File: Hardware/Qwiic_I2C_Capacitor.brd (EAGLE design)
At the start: 25.4 x 25.4 mm, 38 parts, among them J2 QWIIC_RIGHT_ANGLE, J3 PTH, J4 QWIIC_RIGHT_ANGLE, U1 NCD2400MDFN

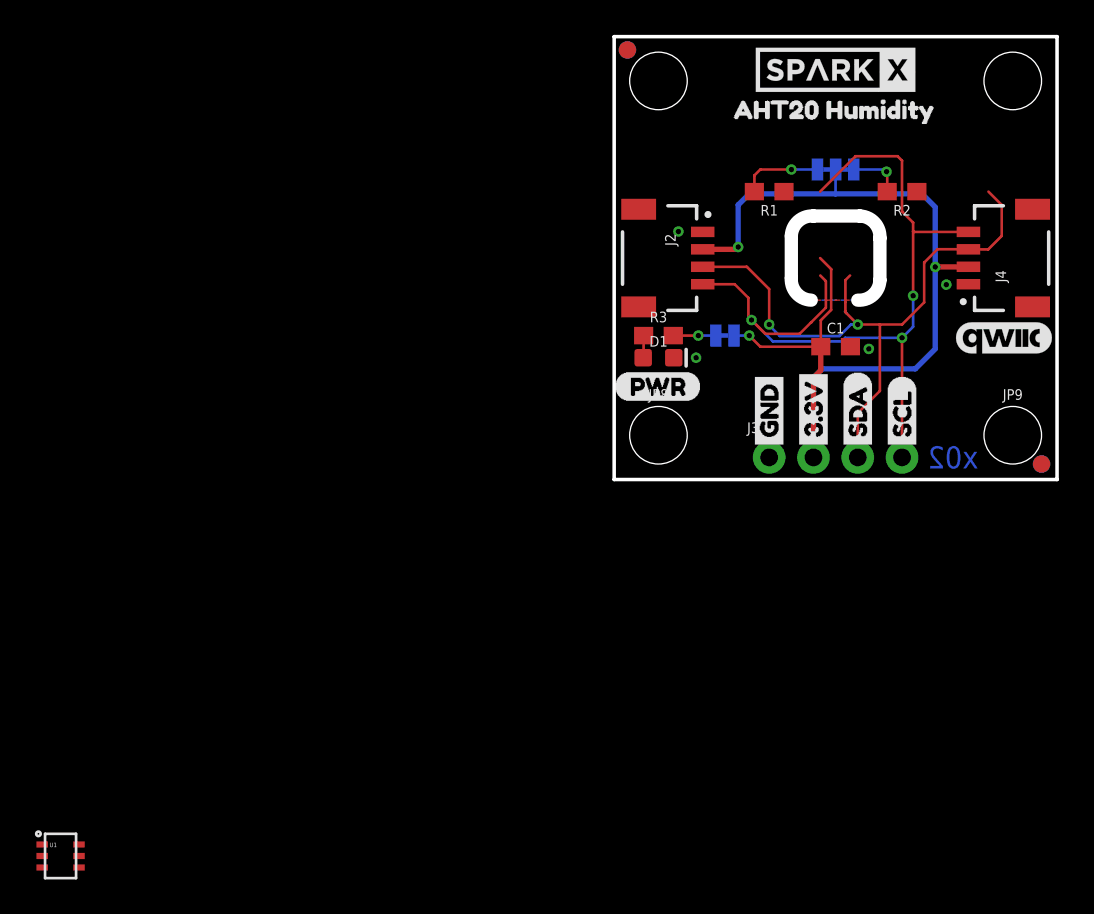
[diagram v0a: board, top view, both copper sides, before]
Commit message: Initial layout
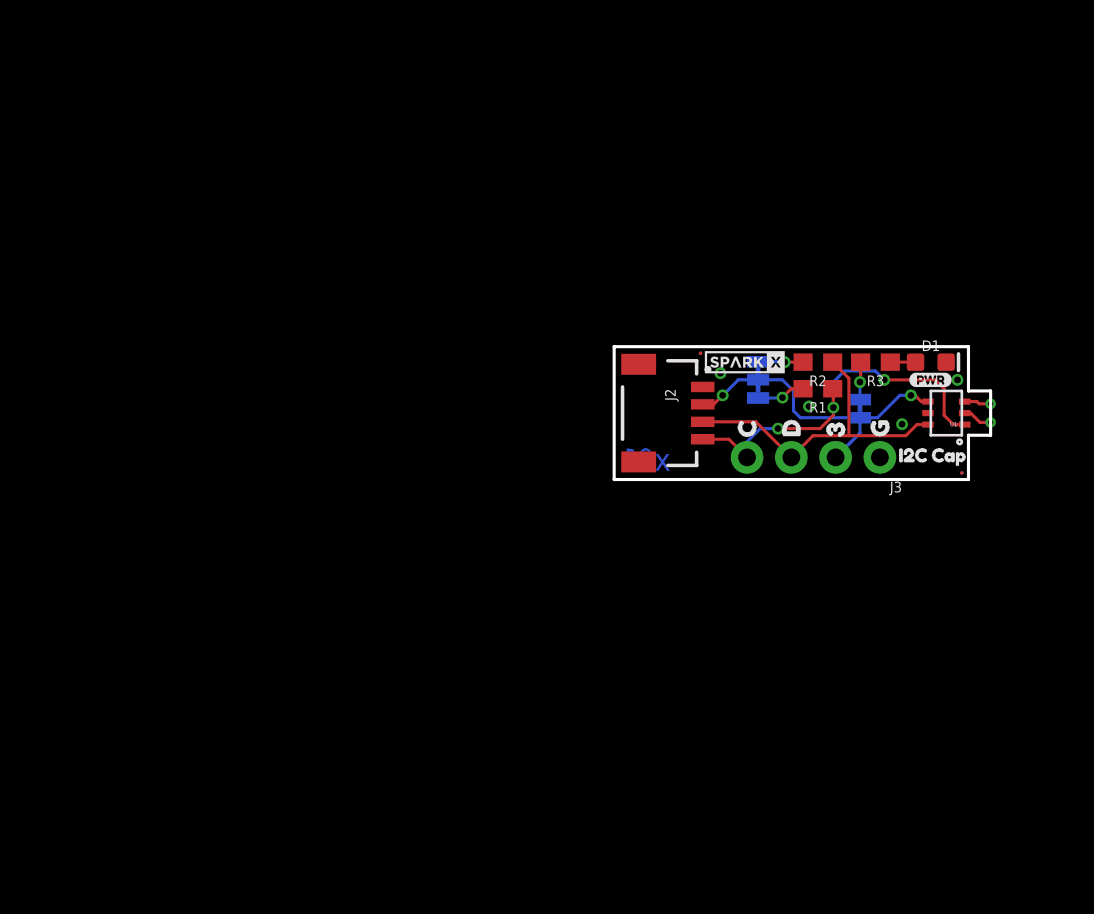
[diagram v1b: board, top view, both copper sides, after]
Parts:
- removed C1: 0.1uF, SparkFun-Capacitors:0603
- removed J4: QWIIC_RIGHT_ANGLE, SparkFun-Connectors:JST04_1MM_RA
- removed JP3, JP4, JP8, JP9: STAND-OFF, SparkFun-Hardware:STAND-OFF
- removed U$11: (no value), SparkFun-Aesthetics:QWIIC_5.5MM
- removed U$22: (no value), Labels-0_04:GND1
- removed U$26: (no value), Labels-0_04:SCL9
- removed U$27: (no value), Labels-0_04:SDA8
- added J1: CONN_02_0603, Qwiic_Capacitor:0603_CASTELLATED
- added U$13: (no value), buzzard_labels (81):D1
- added U$15: (no value), buzzard_labels (83):LED0
- added U$16: (no value), SparkX:SPARKX-TINY
- added U$17: (no value), buzzard_labels (86):CAP1
- added U$19: (no value), buzzard_labels (86):I2C0
- added U$20: (no value), Labels:QWIIC_COPYRIGHT_SMALL
- added U$7: (no value), buzzard_labels (81):32
- JP1, JP2, JP5, JP6: value FIDUCIAL1X2 -> FIDUCIAL0.2MM; device SparkFun-Aesthetics:FIDUCIAL-1X2 -> SparkFun-Aesthetics:FIDUCIAL-0.2MM
- U$1: value SPARKX-LOGO4 -> (none); device SparkX:SPARKX-MEDIUM -> buzzard_labels (86):I2C0
- U$10: device Labels-0_04:(PWR) -> buzzard_labels (85):PWR0
- U$12: device SparkFun-Buzzard:LED_32 -> SparkX:SPARKX-TINY
- U$14: device buzzard_labels (17):AHT20_HUMIDITY2 -> buzzard_labels (81):G3
- U$2: value SPARKX-LOGO4 -> (none); device SparkX:SPARKX-MEDIUM -> buzzard_labels (86):CAP1
- U$21: device Labels-0_04:3#3V2 -> Labels:QWIIC_COPYRIGHT_SMALL
- U$3: device Labels-0_04:GND1 -> buzzard_labels (81):32
- U$4: device Labels-0_04:3#3V2 -> buzzard_labels (81):C0
- U$5: device Labels-0_04:SDA8 -> buzzard_labels (81):D1
- U$6: device Labels-0_04:SCL9 -> buzzard_labels (81):G3
- U$8: device buzzard_labels (17):AHT20_HUMIDITY2 -> buzzard_labels (81):C0
- moved U1 56.8 mm to (19.1, 3.81), turned to 180 degrees
- moved U$8 22.9 mm to (7.62, 1.52), flipped to the top, turned to 90 degrees
- moved U$2 22.6 mm to (17.5, 1.40), flipped to the top
- moved U$1 22.3 mm to (15.6, 1.40)
- moved U$14 21.8 mm to (15.2, 1.52), turned to 90 degrees
- moved JP1 17.9 mm to (4.95, 7.24)
- moved JP6 17.9 mm to (4.95, 7.24)
- moved U$10 16.9 mm to (16.9, 5.71)
- moved U$9 15.9 mm to (10.2, 4.32), turned to 90 degrees
- moved D1 15.6 mm to (18.2, 6.73)
- moved JP7 12.9 mm to (8.26, 5.71), turned to 270 degrees
- moved R3 12.5 mm to (15.0, 6.73), turned to 180 degrees
- moved R1 11.6 mm to (11.7, 5.21)
- moved R2 10.9 mm to (11.7, 6.73)
- moved U$21 10.4 mm to (1.27, 3.81), flipped to the bottom
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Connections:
- new net CN: J1.P$2, U1.3
- new net CP: J1.P$1, U1.2
- net 3.3V: no longer C1.1, J4.2
- net GND: no longer C1.2, J4.1
- net SCL: no longer J4.4
- net SDA: no longer J4.3
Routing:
- net 3.3V: track 57.4 -> 18.6 mm, vias 3 -> 2
- net SCL: track 47.1 -> 22.4 mm
- net SDA: track 38.0 -> 19.1 mm, vias 2 -> 0
- net N$1: track 4.69 -> 2.80 mm
- net CP: track 0.00 -> 1.71 mm
- net CN: track 0.00 -> 1.54 mm
- net N$2: track 3.09 -> 2.59 mm
- removed copper zone on layer 1, net N$6
- removed copper zone on layer 16, net N$6
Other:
- board size 25.4 x 25.4 mm -> 21.6 x 7.6 mm
- board text added: "x01"
- board text removed: "x02"
